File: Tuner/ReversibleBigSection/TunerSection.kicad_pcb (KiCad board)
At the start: 2 copper layers, 100 x 100 mm, 118 parts, among them J1 Conn_01x03, J10 Conn_01x02, J11 Conn_02x05_Odd_Even, J12 Conn_01x01, J13 Conn_01x01, J14 Conn_01x01, J15 Conn_01x01, J16 Conn_01x01, J17 Conn_01x01, J18 Conn_01x01, J19 Conn_01x01, J2 Conn_01x03, J20 Conn_01x01, J21 Conn_01x01, J22 Conn_01x01, J3 Conn_01x03, J4 Conn_01x03, J5 Conn_01x03, J6 Conn_01x03, J7 Conn_01x03, J8 Conn_01x02, J9 Conn_01x02, P10 Conn_01x01, P11 Conn_01x01, P12 Conn_01x01, P2 Conn_01x01, P3 Conn_01x01, P4 Conn_01x01, P5 Conn_01x01, P6 Conn_01x01, P7 Conn_01x01, P8 Conn_01x01, P9 Conn_01x01, U1 MCP23008, U2 ULN2803A

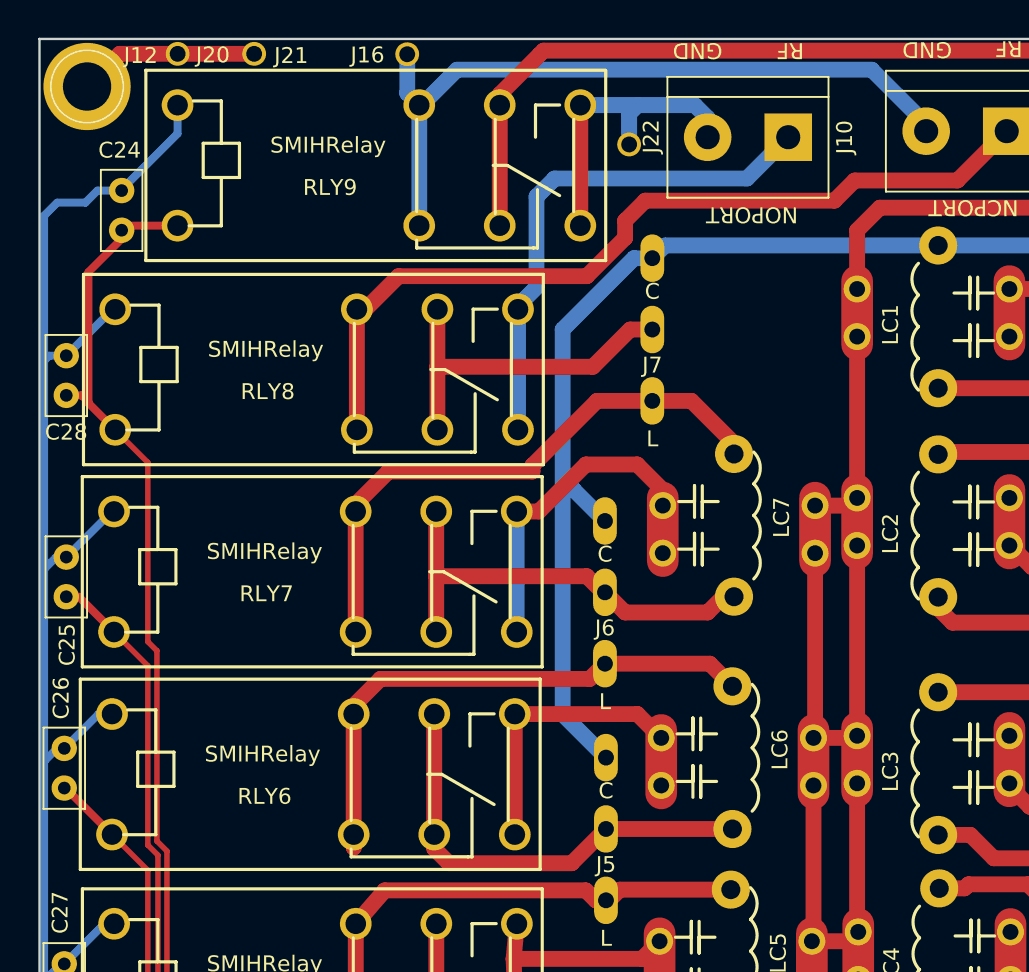
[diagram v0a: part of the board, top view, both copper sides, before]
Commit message: First code commit
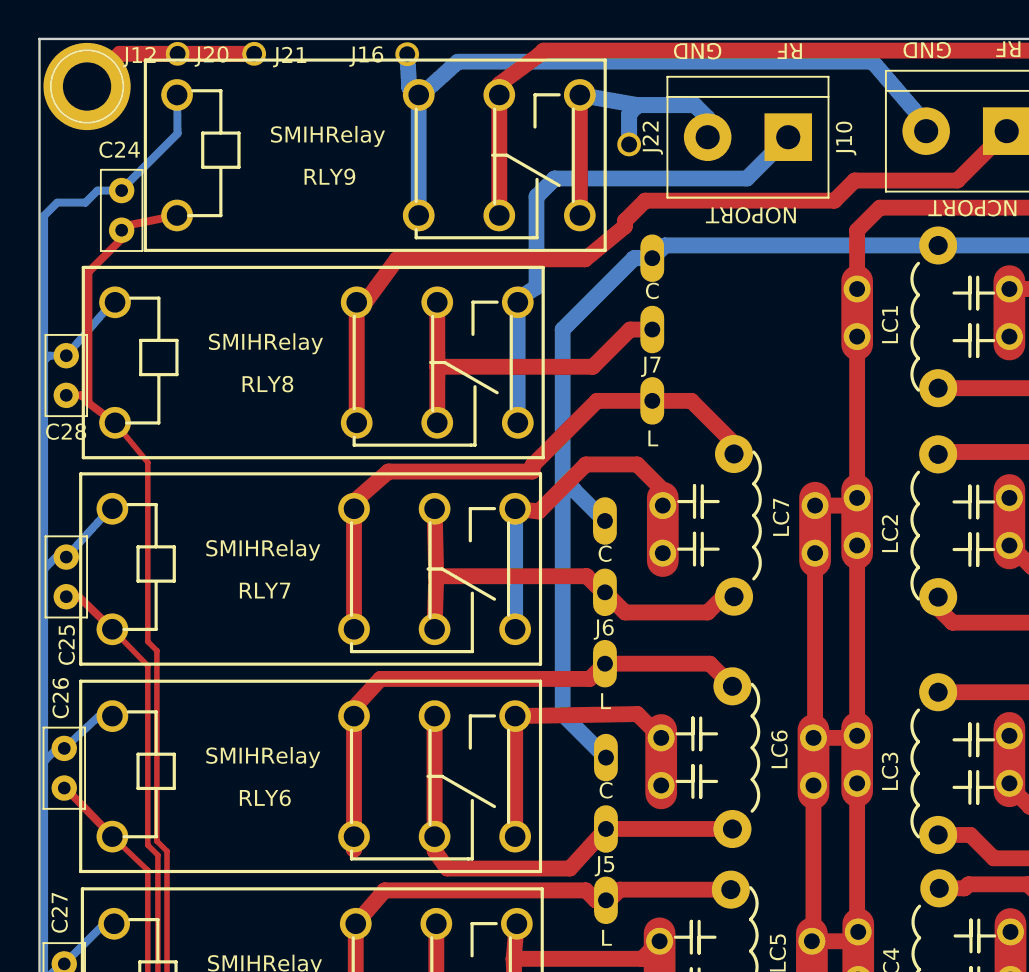
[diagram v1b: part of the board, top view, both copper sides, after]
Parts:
- moved RLY9 0.64 mm to (68.7, 57.3)
- moved RLY8 0.44 mm to (64.8, 70.4)
- moved RLY7 0.20 mm to (64.6, 83.4)
- moved RLY6 0.13 mm to (64.6, 96.5)
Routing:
- net RLYPWR: track 358.8 -> 359.8 mm
